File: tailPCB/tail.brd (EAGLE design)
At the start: 63.2 x 30.5 mm, 6 parts

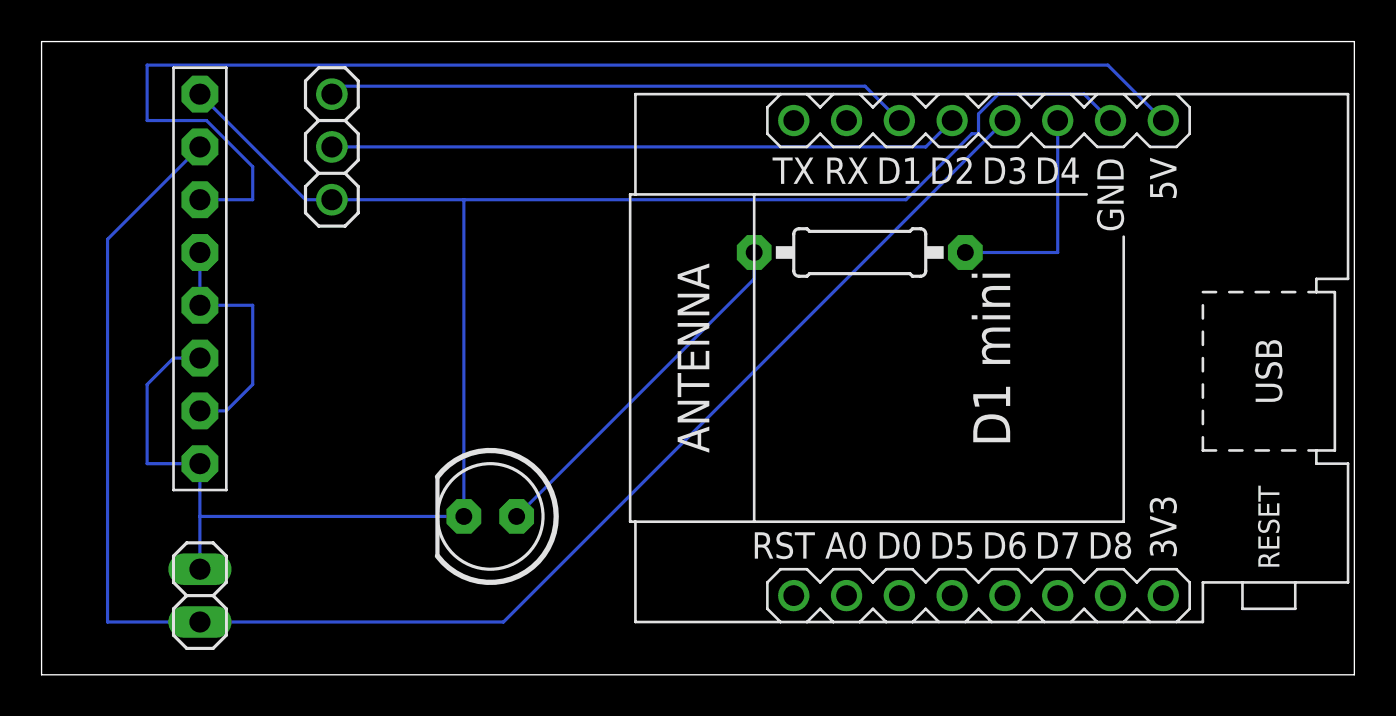
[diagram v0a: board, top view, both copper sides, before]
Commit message: Add files via upload
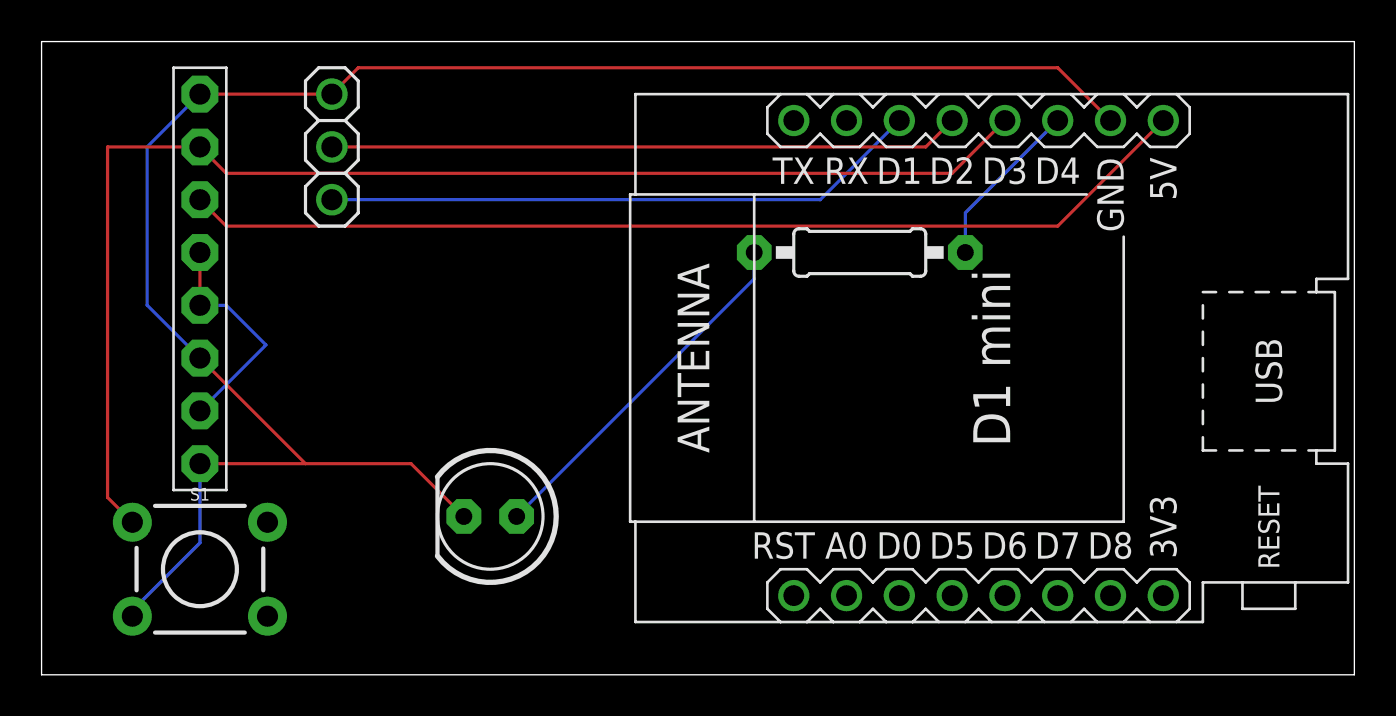
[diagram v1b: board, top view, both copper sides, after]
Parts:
- removed JP3: (no value), DC_LOAD_AU:1X02
- added S1: MOMENTARY-SWITCH-SPST-PTH-6.0MM, SparkFun-Switches:TACTILE_SWITCH_PTH_6.0MM
- turned JP2 to 270 degrees
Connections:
- net 0: now also S1.3; no longer JP3.2
- net N$10: now also S1.1; no longer JP3.1
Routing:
- net N$10: track 77.9 -> 63.3 mm
- net N$6: track 62.8 -> 49.0 mm
- net N$8: track 10.8 -> 8.19 mm
- net 0: track 91.5 -> 89.8 mm
- net N$4: track 12.0 -> 11.0 mm
- net N$3: track 28.1 -> 28.9 mm
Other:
- board text added: "D1 D2 G"
- board text added: "G +5 G +5 JMP BTN"
- board text removed: "BTN JMP +5 G +5 G"
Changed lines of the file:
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@@
 <drawing>
 <settings>
-<setting alwaysvectorfont="yes"/>
+<setting alwaysvectorfont="no"/>
 <setting verticaltext="up"/>
 </settings>
@@
 <wire x1="63.17" y1="80" x2="0" y2="80" width="0" layer="20"/>
 <wire x1="0" y1="80" x2="0" y2="49.53" width="0" layer="20"/>
-<text x="2.413" y="77.724" size="1.27" layer="27" rot="R270">BTN   JMP  +5 G +5 G</text>
+<text x="2.794" y="77.597" size="1.27" layer="27" rot="R270">G +5  G +5    JMP  BTN</text>
+<text x="15.875" y="77.978" size="1.27" layer="27" rot="R270">D1 D2 G</text>
 </plain>
 <attributes>
@@
 <param name="TopRouterVariant" value="1"/>
 <param name="tpViaShape" value="round"/>
-<param name="PrefDir.1" value="0"/>
+<param name="PrefDir.1" value="a"/>
 <param name="PrefDir.2" value="0"/>
 <param name="PrefDir.3" value="0"/>
@@
 <attribute name="VALUE" x="37.1094" y="69.215" size="1.27" layer="27" ratio="10"/>
 </element>
-<element name="JP3" library="DC_LOAD_AU" library_urn="urn:adsk.eagle:library:220454" package="1X02" package3d_urn="urn:adsk.eagle:package:220539/2" value="" x="7.62" y="53.34" smashed="yes" rot="R90">
-<attribute name="VALUE" x="10.795" y="50.8" size="1.27" layer="27" rot="R90"/>
+<element name="JP2" library="adafruit" library_urn="urn:adsk.eagle:library:420" package="1X03" package3d_urn="urn:adsk.eagle:package:6240710/1" value="" x="13.97" y="74.93" smashed="yes" rot="R270">
+<attribute name="VALUE" x="10.795" y="78.74" size="1.27" layer="27" rot="R270"/>
 </element>
-<element name="JP2" library="adafruit" library_urn="urn:adsk.eagle:library:420" package="1X03" package3d_urn="urn:adsk.eagle:package:6240710/1" value="" x="13.97" y="74.93" smashed="yes" rot="R90">
-<attribute name="VALUE" x="17.145" y="71.12" size="1.27" layer="27" rot="R90"/>
+<element name="S1" library="SparkFun-Switches" library_urn="urn:adsk.eagle:library:535" package="TACTILE_SWITCH_PTH_6.0MM" package3d_urn="urn:adsk.eagle:package:40163/1" value="MOMENTARY-SWITCH-SPST-PTH-6.0MM" x="7.62" y="54.61" smashed="yes">
+<attribute name="NAME" x="7.62" y="57.912" size="0.6096" layer="25" font="vector" ratio="20" align="bottom-center"/>
+<attribute name="PROD_ID" value=" SWCH-08441" x="7.62" y="54.61" size="1.778" layer="27" display="off"/>
+<attribute name="SF_SKU" value="COM-00097" x="7.62" y="54.61" size="1.778" layer="27" display="off"/>
+<attribute name="VALUE" x="7.62" y="51.435" size="0.6096" layer="27" font="vector" ratio="20" align="top-center" display="off"/>
 </element>
 </elements>
@@
 <signal name="0">
 <contactref element="LED3" pad="K"/>
-<contactref element="JP3" pad="2"/>
 <contactref element="JP2" pad="1"/>
 <contactref element="W1" pad="JP2.7"/>
@@
 <contactref element="JP1" pad="3"/>
 <contactref element="JP1" pad="8"/>
-<wire x1="7.62" y1="59.69" x2="7.62" y2="57.15" width="0.1524" layer="16"/>
-<wire x1="7.62" y1="57.15" x2="7.62" y2="54.61" width="0.1524" layer="16"/>
-<wire x1="7.62" y1="57.15" x2="20.32" y2="57.15" width="0.1524" layer="16"/>
-<wire x1="6.35" y1="64.77" x2="7.62" y2="64.77" width="0.1524" layer="16"/>
-<wire x1="6.35" y1="64.77" x2="5.08" y2="63.5" width="0.1524" layer="16"/>
-<wire x1="5.08" y1="59.69" x2="5.08" y2="63.5" width="0.1524" layer="16"/>
-<wire x1="7.62" y1="59.69" x2="5.08" y2="59.69" width="0.1524" layer="16"/>
-<wire x1="50.165" y1="77.47" x2="51.435" y2="76.2" width="0.1524" layer="16"/>
-<wire x1="46.0375" y1="77.47" x2="50.165" y2="77.47" width="0.1524" layer="16"/>
-<wire x1="45.085" y1="76.5175" x2="46.0375" y2="77.47" width="0.1524" layer="16"/>
-<wire x1="45.085" y1="75.565" x2="45.085" y2="76.5175" width="0.1524" layer="16"/>
-<wire x1="44.7675" y1="75.565" x2="45.085" y2="75.565" width="0.1524" layer="16"/>
-<wire x1="41.5925" y1="72.39" x2="44.7675" y2="75.565" width="0.1524" layer="16"/>
-<wire x1="13.97" y1="72.39" x2="20.32" y2="72.39" width="0.1524" layer="16"/>
-<wire x1="20.32" y1="72.39" x2="41.5925" y2="72.39" width="0.1524" layer="16"/>
-<wire x1="12.7" y1="72.39" x2="7.62" y2="77.47" width="0.1524" layer="16"/>
-<wire x1="13.97" y1="72.39" x2="12.7" y2="72.39" width="0.1524" layer="16"/>
-<wire x1="20.32" y1="72.39" x2="20.32" y2="57.15" width="0.1524" layer="16"/>
+<contactref element="S1" pad="3"/>
+<wire x1="17.78" y1="59.69" x2="20.32" y2="57.15" width="0.1524" layer="1"/>
+<wire x1="7.62" y1="59.69" x2="12.7" y2="59.69" width="0.1524" layer="1"/>
+<wire x1="12.7" y1="59.69" x2="17.78" y2="59.69" width="0.1524" layer="1"/>
+<wire x1="12.7" y1="59.69" x2="7.62" y2="64.77" width="0.1524" layer="1"/>
+<wire x1="7.62" y1="55.88" x2="4.445" y2="52.705" width="0.1524" layer="16"/>
+<wire x1="7.62" y1="59.69" x2="7.62" y2="55.88" width="0.1524" layer="16"/>
+<wire x1="4.445" y1="52.705" x2="4.3688" y2="52.3494" width="0.1524" layer="16"/>
+<wire x1="48.895" y1="78.74" x2="51.435" y2="76.2" width="0.1524" layer="1"/>
+<wire x1="48.895" y1="78.74" x2="15.24" y2="78.74" width="0.1524" layer="1"/>
+<wire x1="13.97" y1="77.47" x2="15.24" y2="78.74" width="0.1524" layer="1"/>
+<wire x1="13.97" y1="77.47" x2="7.62" y2="77.47" width="0.1524" layer="1"/>
+<wire x1="5.08" y1="67.31" x2="7.62" y2="64.77" width="0.1524" layer="16"/>
+<wire x1="5.08" y1="74.93" x2="5.08" y2="67.31" width="0.1524" layer="16"/>
+<wire x1="7.62" y1="77.47" x2="5.08" y2="74.93" width="0.1524" layer="16"/>
 </signal>
 <signal name="N$8">
 <contactref element="R4" pad="2"/>
 <contactref element="W1" pad="JP2.6"/>
-<wire x1="48.895" y1="69.85" x2="48.895" y2="76.2" width="0.1524" layer="16"/>
-<wire x1="44.45" y1="69.85" x2="48.895" y2="69.85" width="0.1524" layer="16"/>
+<wire x1="44.45" y1="71.755" x2="48.895" y2="76.2" width="0.1524" layer="16"/>
+<wire x1="44.45" y1="69.85" x2="44.45" y2="71.755" width="0.1524" layer="16"/>
 </signal>
 <signal name="N$9">
@@
 </signal>
 <signal name="N$10">
-<contactref element="JP3" pad="1"/>
 <contactref element="W1" pad="JP2.5"/>
 <contactref element="JP1" pad="7"/>
-<wire x1="22.225" y1="52.07" x2="46.355" y2="76.2" width="0.1524" layer="16"/>
-<wire x1="7.62" y1="52.07" x2="22.225" y2="52.07" width="0.1524" layer="16"/>
-<wire x1="3.175" y1="70.485" x2="7.62" y2="74.93" width="0.1524" layer="16"/>
-<wire x1="3.175" y1="52.07" x2="3.175" y2="70.485" width="0.1524" layer="16"/>
-<wire x1="7.62" y1="52.07" x2="3.175" y2="52.07" width="0.1524" layer="16"/>
+<contactref element="S1" pad="1"/>
+<wire x1="43.815" y1="73.66" x2="46.355" y2="76.2" width="0.1524" layer="1"/>
+<wire x1="8.89" y1="73.66" x2="43.815" y2="73.66" width="0.1524" layer="1"/>
+<wire x1="7.62" y1="74.93" x2="8.89" y2="73.66" width="0.1524" layer="1"/>
+<wire x1="3.175" y1="74.93" x2="3.175" y2="58.0644" width="0.1524" layer="1"/>
+<wire x1="4.3688" y1="56.8706" x2="3.175" y2="58.0644" width="0.1524" layer="1"/>
+<wire x1="7.62" y1="74.93" x2="3.175" y2="74.93" width="0.1524" layer="1"/>
 </signal>
 <signal name="N$2">
 <contactref element="W1" pad="JP2.4"/>
 <contactref element="JP2" pad="2"/>
-<wire x1="42.545" y1="74.93" x2="43.815" y2="76.2" width="0.1524" layer="16"/>
-<wire x1="13.97" y1="74.93" x2="42.545" y2="74.93" width="0.1524" layer="16"/>
+<wire x1="42.545" y1="74.93" x2="43.815" y2="76.2" width="0.1524" layer="1"/>
+<wire x1="13.97" y1="74.93" x2="42.545" y2="74.93" width="0.1524" layer="1"/>
 </signal>
 <signal name="N$3">
 <contactref element="W1" pad="JP2.3"/>
 <contactref element="JP2" pad="3"/>
-<wire x1="39.624" y1="77.851" x2="41.275" y2="76.2" width="0.1524" layer="16"/>
-<wire x1="39.624" y1="77.851" x2="14.351" y2="77.851" width="0.1524" layer="16"/>
-<wire x1="13.97" y1="77.47" x2="14.351" y2="77.851" width="0.1524" layer="16"/>
+<wire x1="37.465" y1="72.39" x2="41.275" y2="76.2" width="0.1524" layer="16"/>
+<wire x1="13.97" y1="72.39" x2="37.465" y2="72.39" width="0.1524" layer="16"/>
 </signal>
 <signal name="N$4">
@@
 <contactref element="JP1" pad="4"/>
 <contactref element="JP1" pad="5"/>
-<wire x1="10.16" y1="63.5" x2="8.89" y2="62.23" width="0.1524" layer="16"/>
-<wire x1="8.89" y1="62.23" x2="7.62" y2="62.23" width="0.1524" layer="16"/>
-<wire x1="10.16" y1="67.31" x2="10.16" y2="63.5" width="0.1524" layer="16"/>
-<wire x1="7.62" y1="67.31" x2="10.16" y2="67.31" width="0.1524" layer="16"/>
-<wire x1="7.62" y1="67.31" x2="7.62" y2="69.85" width="0.1524" layer="16"/>
+<wire x1="10.795" y1="65.405" x2="7.62" y2="62.23" width="0.1524" layer="16"/>
+<wire x1="10.795" y1="65.405" x2="8.89" y2="67.31" width="0.1524" layer="16"/>
+<wire x1="7.62" y1="67.31" x2="8.89" y2="67.31" width="0.1524" layer="16"/>
+<wire x1="7.62" y1="67.31" x2="7.62" y2="69.85" width="0.1524" layer="1"/>
 </signal>
 <signal name="N$6">
 <contactref element="JP1" pad="6"/>
 <contactref element="W1" pad="JP2.8"/>
-<wire x1="51.308" y1="78.867" x2="53.975" y2="76.2" width="0.1524" layer="16"/>
-<wire x1="5.08" y1="78.867" x2="51.308" y2="78.867" width="0.1524" layer="16"/>
-<wire x1="5.08" y1="76.2" x2="5.08" y2="78.867" width="0.1524" layer="16"/>
-<wire x1="7.9375" y1="76.2" x2="5.08" y2="76.2" width="0.1524" layer="16"/>
-<wire x1="10.16" y1="73.9775" x2="7.9375" y2="76.2" width="0.1524" layer="16"/>
-<wire x1="10.16" y1="72.39" x2="10.16" y2="73.9775" width="0.1524" layer="16"/>
-<wire x1="7.62" y1="72.39" x2="10.16" y2="72.39" width="0.1524" layer="16"/>
+<wire x1="48.895" y1="71.12" x2="53.975" y2="76.2" width="0.1524" layer="1"/>
+<wire x1="8.89" y1="71.12" x2="48.895" y2="71.12" width="0.1524" layer="1"/>
+<wire x1="7.62" y1="72.39" x2="8.89" y2="71.12" width="0.1524" layer="1"/>
 </signal>
 </signals>
